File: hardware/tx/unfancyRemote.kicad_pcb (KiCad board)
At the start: 2 copper layers, 23.9 x 37 mm, 57 parts, among them J1 Battery, J3 HALL1/PPM, J4 HALL2, J6 VIN, J8 Motor, Q1 AO3401A, Q2 MMBT3904, Q3 MMBT3904, SW1 SW_Push, U1 E28-2G4M12S, U2 MCP73871-2AA, U3 ESP32-C3_SUPERMINI, U4 TPS61085DGK, U5 MIC5219-3.3YM5

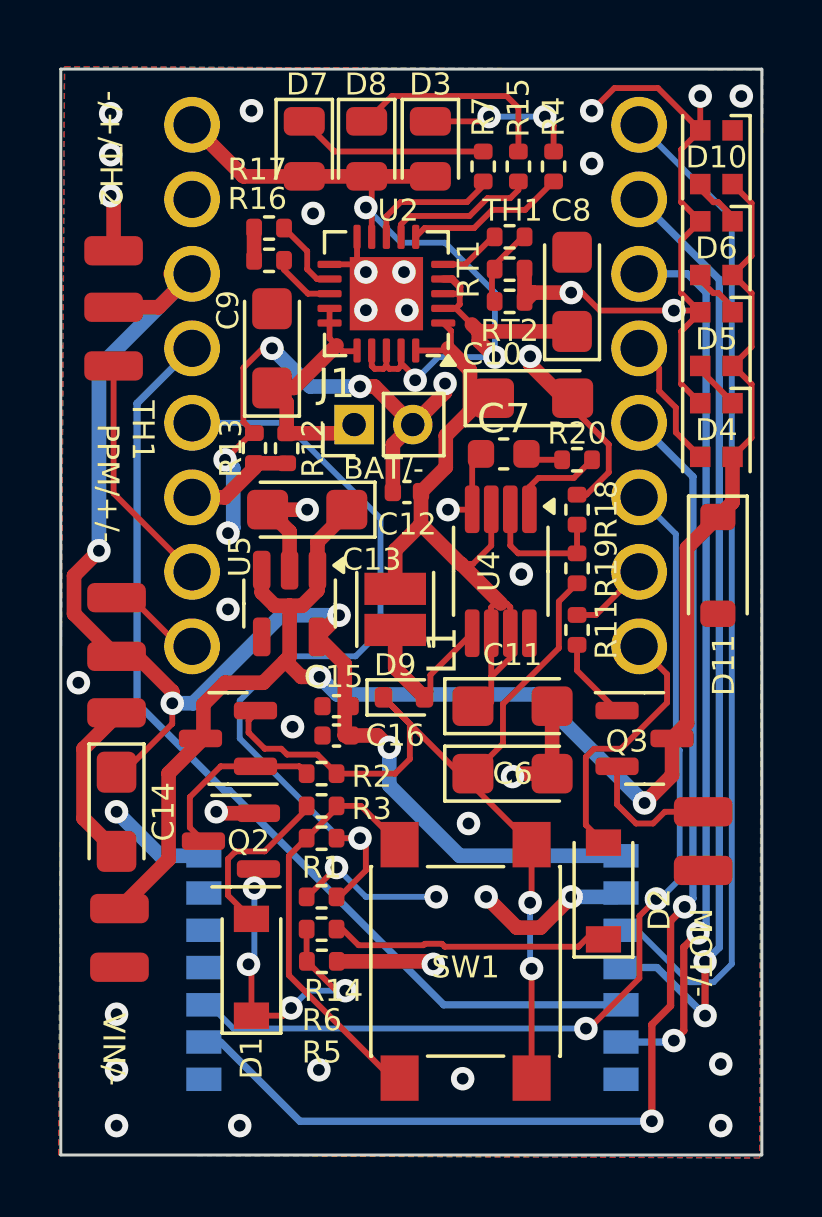
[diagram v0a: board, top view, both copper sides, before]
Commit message: optimize all the things
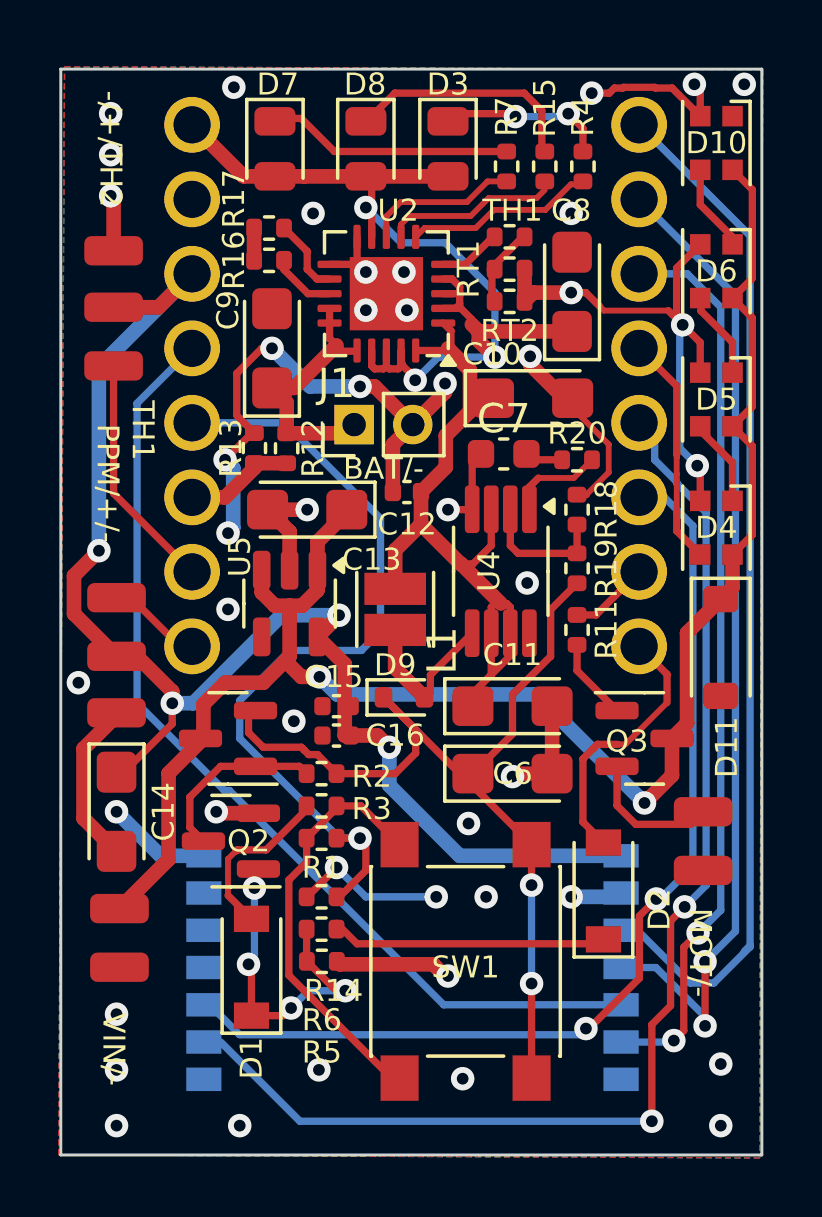
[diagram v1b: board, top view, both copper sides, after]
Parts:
- moved D4 3.33 mm to (143.3, 79.4)
- moved D11 2.80 mm to (143.5, 83.5)
- moved D5 2.06 mm to (143.3, 75.0)
- moved D7 1.00 mm to (128.3, 66.5)
- moved R4 1.00 mm to (138.8, 67.1)
- moved R15 0.90 mm to (137.5, 67.1)
- moved R7 0.80 mm to (136.2, 67.1)
- moved D6 0.79 mm to (143.3, 70.7)
- moved D3 0.60 mm to (134.2, 66.5)
- moved D10 0.48 mm to (143.3, 66.3)
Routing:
- net GND: track 88.6 -> 84.6 mm, vias 44 -> 45
- net LED: track 4.56 -> 7.90 mm
- net Net-(D7-K): track 6.53 -> 8.37 mm
- net +3V3: track 48.9 -> 47.2 mm
- net Net-(D10-DIN): track 1.49 -> 3.00 mm
- net Net-(D5-DOUT): track 1.49 -> 2.96 mm
- net Net-(D4-DOUT): track 1.56 -> 2.86 mm
- net /MOSI: track 32.7 -> 33.8 mm
- net /RFBUSY: track 33.3 -> 34.4 mm
- net Net-(U2-STAT1/~{LBO}): track 4.43 -> 5.29 mm
- net Net-(U2-~{PG}): track 5.48 -> 6.34 mm
- net /MISO: track 34.7 -> 35.5 mm
- net Net-(D8-K): track 7.19 -> 7.91 mm
- net VBAT: track 9.34 -> 8.68 mm
- net Net-(U2-STAT2): track 5.21 -> 5.81 mm
